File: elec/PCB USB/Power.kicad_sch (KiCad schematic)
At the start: 23 parts, among them Q301 AO3401A, U301 AP7361C-33E

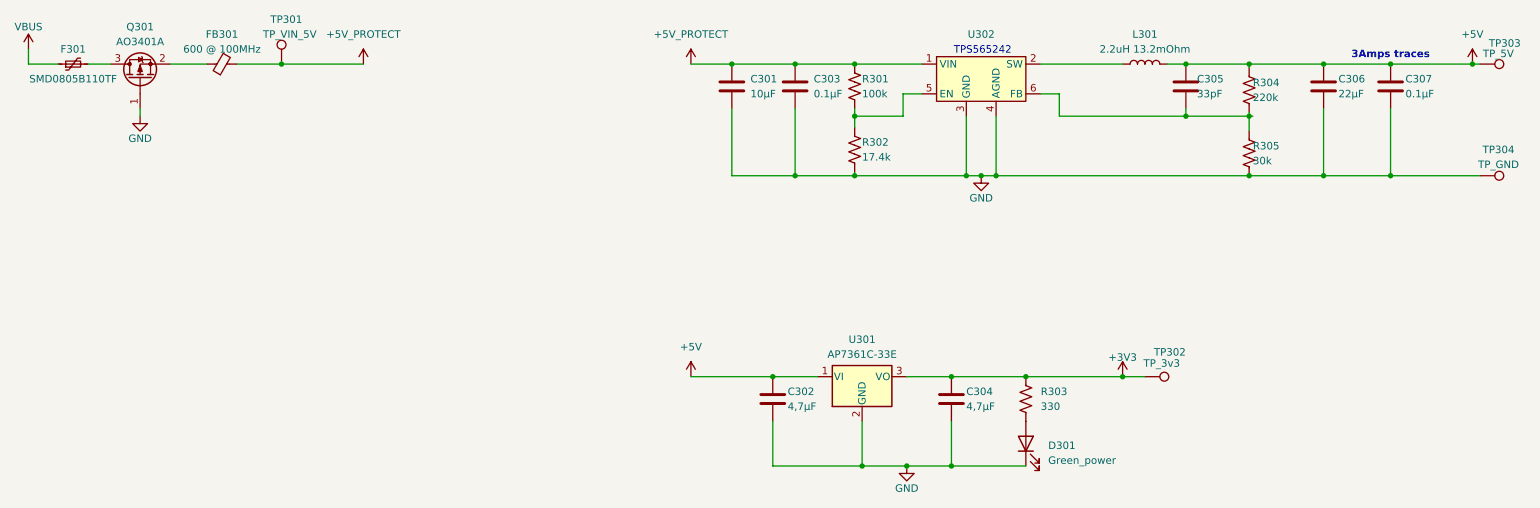
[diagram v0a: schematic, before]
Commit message: push pcb
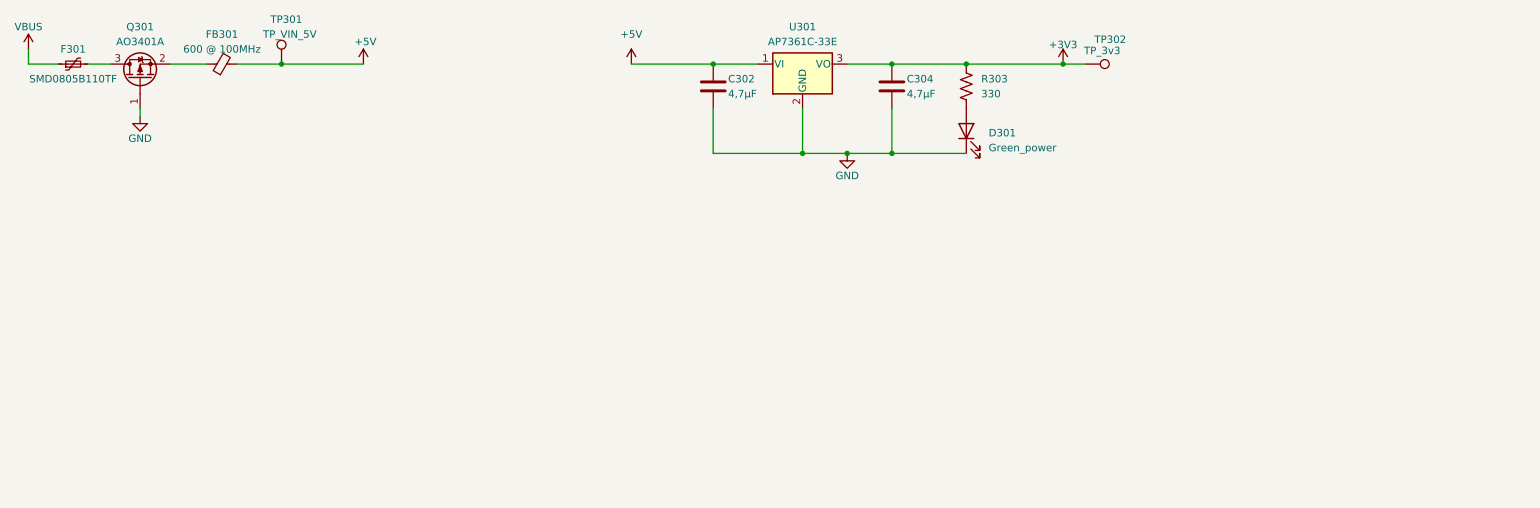
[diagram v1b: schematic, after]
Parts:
- removed C301: 10µF, Capacitor_SMD:C_0805_2012Metric_Pad1.18x1.45mm_HandSolder, symbol Device:C
- removed C303, C307: 0.1µF, Capacitor_SMD:C_0603_1608Metric_Pad1.08x0.95mm_HandSolder, symbol Device:C
- removed C305: 33pF, Capacitor_SMD:C_0603_1608Metric_Pad1.08x0.95mm_HandSolder, symbol Device:C
- removed C306: 22µF, Capacitor_SMD:C_0805_2012Metric_Pad1.18x1.45mm_HandSolder, symbol Device:C
- removed L301: 2.2uH 13.2mOhm, Inductor_SMD:L_TDK_VLP8040, symbol Device:L
- removed R301: 100k, Resistor_SMD:R_0603_1608Metric_Pad0.98x0.95mm_HandSolder, symbol Device:R_US
- removed R302: 17.4k, Resistor_SMD:R_0603_1608Metric_Pad0.98x0.95mm_HandSolder, symbol Device:R_US
- removed R304: 220k, Resistor_SMD:R_0603_1608Metric_Pad0.98x0.95mm_HandSolder, symbol Device:R_US
- removed R305: 30k, Resistor_SMD:R_0603_1608Metric_Pad0.98x0.95mm_HandSolder, symbol Device:R_US
- removed TP303: TP_5V, TestPoint:TestPoint_Pad_D1.0mm, symbol Connector:TestPoint
- removed TP304: TP_GND, TestPoint:TestPoint_Pad_1.0x1.0mm, symbol Connector:TestPoint
- removed U302: ~, Package_TO_SOT_SMD:SOT-563, symbol TPS565242:TPS565242
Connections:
- net +5V_PROTECT is gone; now on net +5V: FB301.2, TP301.1
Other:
- note removed: "3Amps traces"
- note removed: "TPS565242"
- moved on the sheet: C302, C304, D301, R303, TP302, U301

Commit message: Push non terminé
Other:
- company: (none) -> C3I
- title: (none) -> Hub USB2.0 Pomodoro
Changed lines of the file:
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@@
 	(generator_version "9.0")
 	(paper "A4")
+	(title_block
+		(title "Hub USB2.0 Pomodoro")
+		(date "2025-04-20")
+		(rev "1.0")
+		(company "C3I")
+		(comment 1 "Jacob Turcotte")
+		(comment 2 "&")
+		(comment 3 "Charles-Ariel Dion")
+		(comment 4 "Par: Équipe 3")
+	)
 	(junction
 		(at 161.29 40.64)
